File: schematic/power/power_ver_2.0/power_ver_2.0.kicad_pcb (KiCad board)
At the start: 2 copper layers, 5 parts, among them Q1 RFP12N10L, Q2 RFP12N10L, Q3 RFP12N10L, Q4 RFP12N10L, U1 HIP4082IP

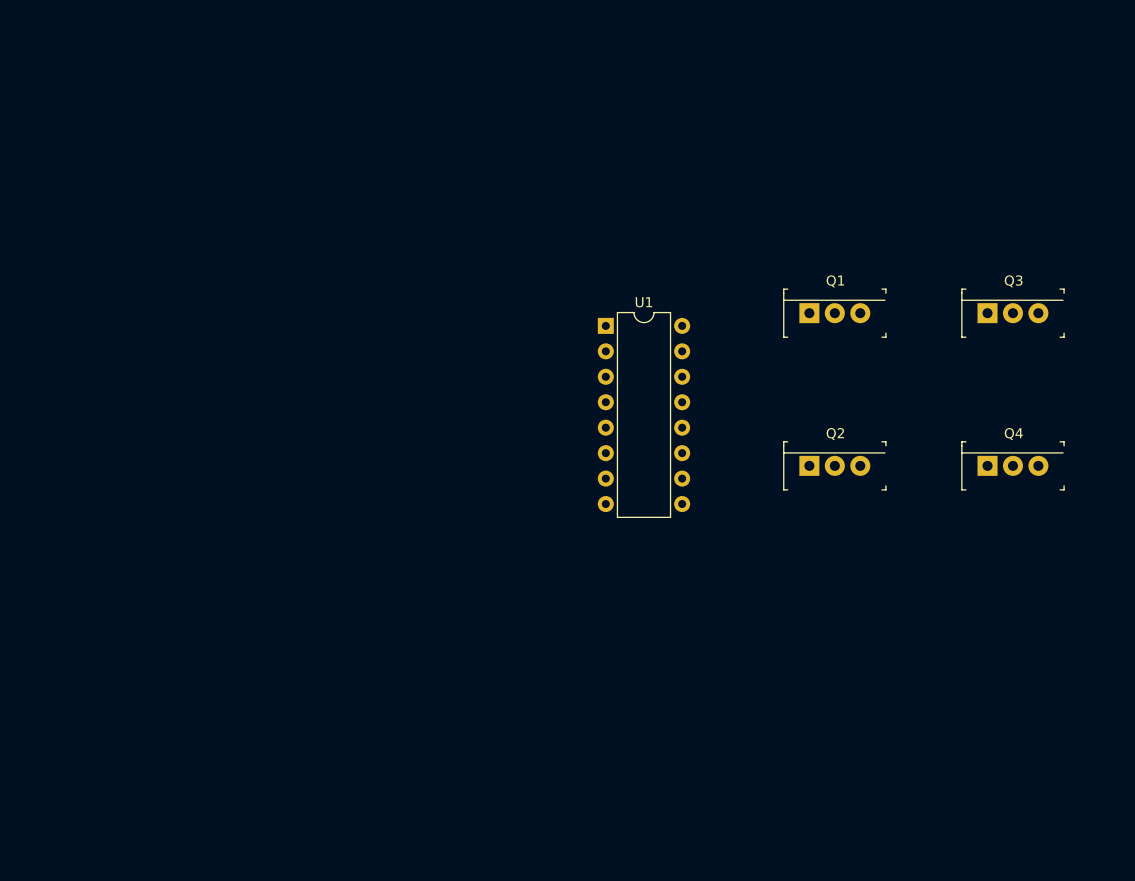
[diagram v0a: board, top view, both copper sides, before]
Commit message: ver2 pcb layout
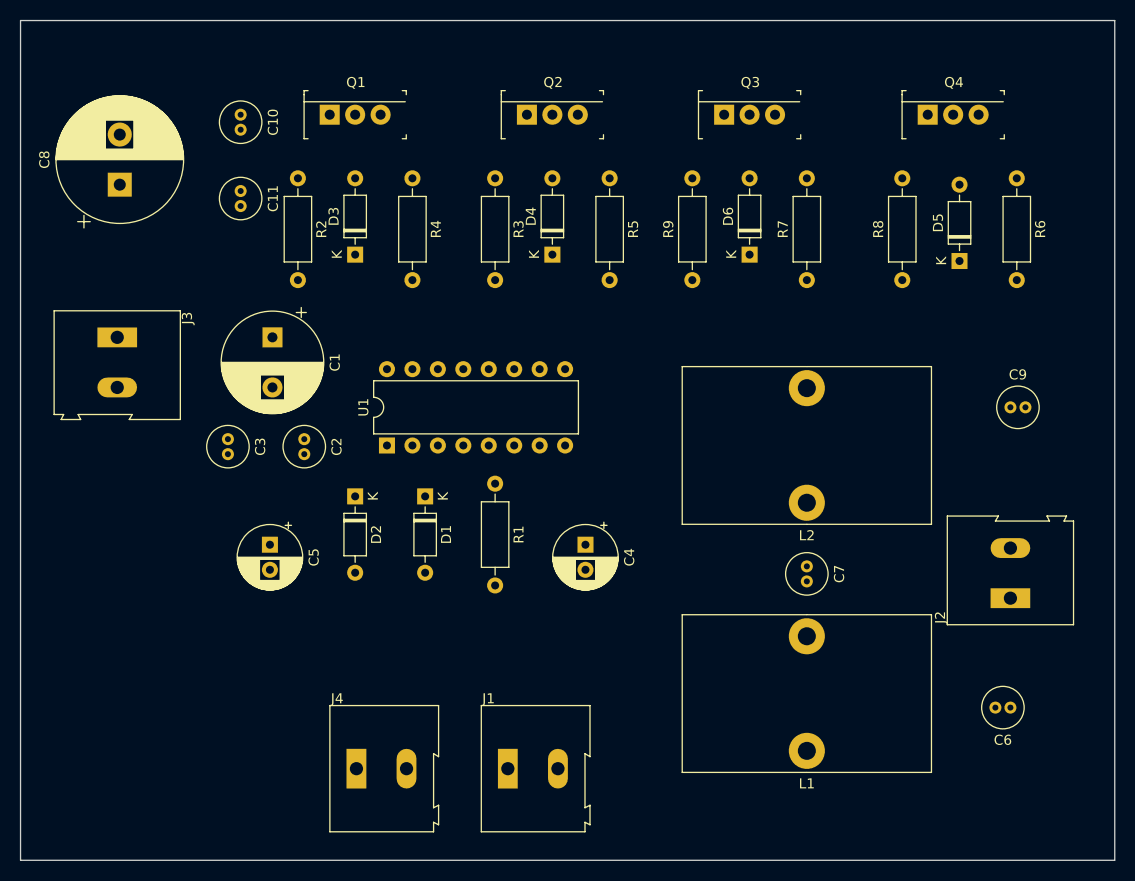
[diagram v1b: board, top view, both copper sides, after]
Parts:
- added C1: ECE-A1HN101U, Capacitor_THT:CP_Radial_D10.0mm_P5.00mm, F.Cu at (109.0, 95.1)
- added C10: C324C106K3R5TA, Capacitor_THT:C_Radial_D4.0mm_H5.0mm_P1.50mm, F.Cu at (105.8, 72.9)
- added C11: SR205C104MAATR1, Capacitor_THT:C_Radial_D4.0mm_H5.0mm_P1.50mm, F.Cu at (105.8, 80.5)
- added C2: C324C106K3R5TA, Capacitor_THT:C_Radial_D4.0mm_H5.0mm_P1.50mm, F.Cu at (112.1, 105.3)
- added C3: SR205C104MAATR1, Capacitor_THT:C_Radial_D4.0mm_H5.0mm_P1.50mm, F.Cu at (104.5, 105.3)
- added C4: ECE-A1HN100U, Capacitor_THT:CP_Radial_D6.3mm_P2.50mm, F.Cu at (140.2, 115.8)
- added C5: ECE-A1HN100U, Capacitor_THT:CP_Radial_D6.3mm_P2.50mm, F.Cu at (108.7, 115.8)
- added C6: C324C106K3R5TA, Capacitor_THT:C_Radial_D4.0mm_H5.0mm_P1.50mm, F.Cu at (182.6, 132.1)
- added C7: C324C106K3R5TA, Capacitor_THT:C_Radial_D4.0mm_H5.0mm_P1.50mm, F.Cu at (162.3, 118.0)
- added C8: EEU-FC1H102L, Capacitor_THT:CP_Radial_D12.5mm_P5.00mm, F.Cu at (93.7, 79.9)
- added C9: C324C106K3R5TA, Capacitor_THT:C_Radial_D4.0mm_H5.0mm_P1.50mm, F.Cu at (182.6, 102.1)
- added D1: 1N4148, Diode_THT:D_DO-35_SOD27_P7.62mm_Horizontal, F.Cu at (124.2, 111.0)
- added D2: 1N4148, Diode_THT:D_DO-35_SOD27_P7.62mm_Horizontal, F.Cu at (117.2, 111.0)
- added D3: 1N4148, Diode_THT:D_DO-35_SOD27_P7.62mm_Horizontal, F.Cu at (117.2, 86.9)
- added D4: 1N4148, Diode_THT:D_DO-35_SOD27_P7.62mm_Horizontal, F.Cu at (136.9, 86.9)
- added D5: 1N4148, Diode_THT:D_DO-35_SOD27_P7.62mm_Horizontal, F.Cu at (177.5, 87.5)
- added D6: 1N4148, Diode_THT:D_DO-35_SOD27_P7.62mm_Horizontal, F.Cu at (156.6, 86.9)
- added J1: PWM INPUT, TerminalBlock:TerminalBlock_Altech_AK300-2_P5.00mm, F.Cu at (132.5, 138.2)
- added J2: Audio OUTPUT, TerminalBlock:TerminalBlock_Altech_AK300-2_P5.00mm, F.Cu at (182.6, 121.2)
- added J3: OUTPUT Power, TerminalBlock:TerminalBlock_Altech_AK300-2_P5.00mm, F.Cu at (93.5, 95.1)
- added J4: PWM_power, TerminalBlock:TerminalBlock_Altech_AK300-2_P5.00mm, F.Cu at (117.3, 138.2)
- added L1: 2216-V-RC, Inductor_THT:L_Toroid_Vertical_L24.6mm_W15.5mm_P11.44mm_Pulse_KM-4, F.Cu at (162.3, 136.4)
- added L2: 2216-V-RC, Inductor_THT:L_Toroid_Vertical_L24.6mm_W15.5mm_P11.44mm_Pulse_KM-4, F.Cu at (162.3, 111.6)
- added R1: 1K, Resistor_THT:R_Axial_DIN0207_L6.3mm_D2.5mm_P10.16mm_Horizontal, F.Cu at (131.2, 109.7)
- added R2: R, Resistor_THT:R_Axial_DIN0207_L6.3mm_D2.5mm_P10.16mm_Horizontal, F.Cu at (111.5, 79.2)
- added R3: R, Resistor_THT:R_Axial_DIN0207_L6.3mm_D2.5mm_P10.16mm_Horizontal, F.Cu at (131.2, 79.2)
- added R4: R, Resistor_THT:R_Axial_DIN0207_L6.3mm_D2.5mm_P10.16mm_Horizontal, F.Cu at (122.9, 79.2)
- added R5: R, Resistor_THT:R_Axial_DIN0207_L6.3mm_D2.5mm_P10.16mm_Horizontal, F.Cu at (142.6, 79.2)
- added R6: R, Resistor_THT:R_Axial_DIN0207_L6.3mm_D2.5mm_P10.16mm_Horizontal, F.Cu at (183.3, 79.2)
- added R7: R, Resistor_THT:R_Axial_DIN0207_L6.3mm_D2.5mm_P10.16mm_Horizontal, F.Cu at (162.3, 89.4)
- added R8: R, Resistor_THT:R_Axial_DIN0207_L6.3mm_D2.5mm_P10.16mm_Horizontal, F.Cu at (171.8, 89.4)
- added R9: R, Resistor_THT:R_Axial_DIN0207_L6.3mm_D2.5mm_P10.16mm_Horizontal, F.Cu at (150.9, 89.4)
- moved Q1 51.8 mm to (114.7, 72.9)
- moved Q2 45.0 mm to (134.4, 72.9)
- moved Q4 35.6 mm to (174.4, 72.9)
- moved Q3 32.9 mm to (154.1, 72.9)
- moved U1 24.9 mm to (120.4, 105.9), turned to 90 degrees
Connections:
- Q1 pad 2: Net-(Q1-Pad2) -> +15V
- Q1 pad 3: Net-(Q1-Pad3) -> Net-(C5-Pad2)
- Q2 pad 2: Net-(Q2-Pad2) -> Net-(C5-Pad2)
- Q2 pad 3: Net-(Q2-Pad3) -> GND
- Q3 pad 2: Net-(Q3-Pad2) -> +15V
- Q3 pad 3: Net-(Q3-Pad3) -> Net-(C4-Pad1)
- Q4 pad 2: Net-(Q4-Pad2) -> Net-(C4-Pad1)
- Q4 pad 3: Net-(Q4-Pad3) -> GND
- U1 pad 11: Net-(U1-Pad11) -> Net-(C4-Pad1)
- U1 pad 12: Net-(U1-Pad12) -> +15V
- U1 pad 15: Net-(U1-Pad15) -> Net-(C5-Pad2)
- U1 pad 2: Net-(U1-Pad2) -> +5V
- U1 pad 3: Net-(U1-Pad3) -> PWM+
- U1 pad 4: Net-(U1-Pad4) -> PWM-
- U1 pad 6: Net-(U1-Pad6) -> GND
- U1 pad 7: Net-(U1-Pad7) -> +5V
- U1 pad 8: Net-(U1-Pad8) -> GND
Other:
- board outline added: 109.2 x 83.8 mm
